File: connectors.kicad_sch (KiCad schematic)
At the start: 4 parts, among them J1 Conn_01x04_Pin, J2 Conn_01x04_Pin, J3 Conn_01x09_Pin, J4 Conn_02x03_Odd_Even

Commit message: Assigned footprints to symbols
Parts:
- J1, J2: footprint (none) -> Connector_PinHeader_2.54mm:PinHeader_1x04_P2.54mm_Vertical
- J3: footprint (none) -> Connector_PinHeader_2.54mm:PinHeader_1x09_P2.54mm_Vertical
- J4: footprint (none) -> Connector_PinHeader_2.54mm:PinHeader_2x03_P2.54mm_Vertical
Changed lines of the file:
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@@
       (effects (font (size 1.27 1.27)))
     )
-    (property "Footprint" "" (at 102.87 105.41 0)
+    (property "Footprint" "Connector_PinHeader_2.54mm:PinHeader_1x09_P2.54mm_Vertical" (at 102.87 105.41 0)
       (effects (font (size 1.27 1.27)) hide)
     )
@@
       (effects (font (size 1.27 1.27)))
     )
-    (property "Footprint" "" (at 101.6 71.12 0)
+    (property "Footprint" "Connector_PinHeader_2.54mm:PinHeader_1x04_P2.54mm_Vertical" (at 101.6 71.12 0)
       (effects (font (size 1.27 1.27)) hide)
     )
@@
       (effects (font (size 1.27 1.27)))
     )
-    (property "Footprint" "" (at 127 71.12 0)
+    (property "Footprint" "Connector_PinHeader_2.54mm:PinHeader_1x04_P2.54mm_Vertical" (at 127 71.12 0)
       (effects (font (size 1.27 1.27)) hide)
     )
@@
       (effects (font (size 1.27 1.27)))
     )
-    (property "Footprint" "" (at 130.81 104.14 0)
+    (property "Footprint" "Connector_PinHeader_2.54mm:PinHeader_2x03_P2.54mm_Vertical" (at 130.81 104.14 0)
       (effects (font (size 1.27 1.27)) hide)
     )

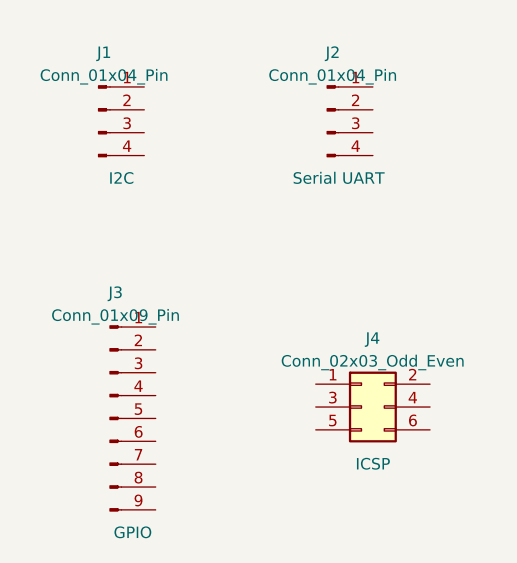
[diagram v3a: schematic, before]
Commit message: completed writing of embedded connector sheet
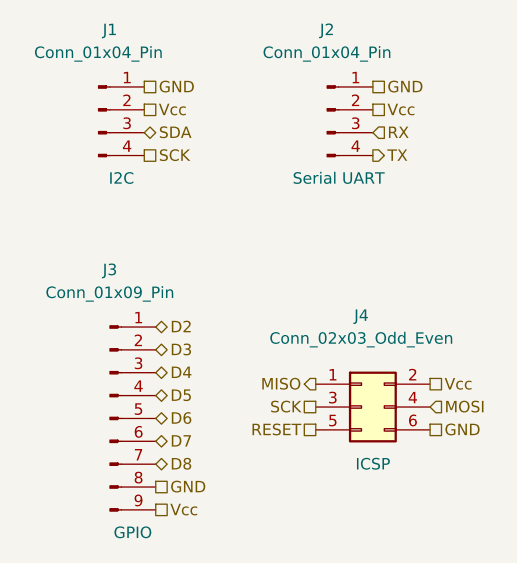
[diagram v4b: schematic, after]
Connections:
- net D2: now reaches J3.1 (Pin_1)
- net D3: now reaches J3.2 (Pin_2)
- net D4: now reaches J3.3 (Pin_3)
- net D5: now reaches J3.4 (Pin_4)
- net D6: now reaches J3.5 (Pin_5)
- net D7: now reaches J3.6 (Pin_6)
- net D8: now reaches J3.7 (Pin_7)
- net GND: now reaches J3.8 (Pin_8)
- net GND: now also J1.1 (Pin_1), J2.1 (Pin_1), J4.6 (Pin_6)
- net Vcc: now reaches J3.9 (Pin_9)
- net Vcc: now also J1.2 (Pin_2), J2.2 (Pin_2), J4.2 (Pin_2)
- net SDA: now reaches J1.3 (Pin_3)
- net SCK: now reaches J1.4 (Pin_4)
- net SCK: now also J4.3 (Pin_3)
- net RX: now reaches J2.3 (Pin_3)
- net TX: now reaches J2.4 (Pin_4)
- net MISO: now reaches J4.1 (Pin_1)
- net MOSI: now reaches J4.4 (Pin_4)
- net RESET: now reaches J4.5 (Pin_5)
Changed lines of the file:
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@@
 (kicad_sch (version 20230121) (generator eeschema)
   (paper "A4")
+  (hierarchical_label "Vcc" (shape passive) (at 106.68 71.12 0) (fields_autoplaced)
+    (effects (font (size 1.27 1.27)) (justify left))
+  )
+  (hierarchical_label "RESET" (shape passive) (at 125.73 106.68 180) (fields_autoplaced)
+    (effects (font (size 1.27 1.27)) (justify right))
+  )
+  (hierarchical_label "Vcc" (shape passive) (at 132.08 71.12 0) (fields_autoplaced)
+    (effects (font (size 1.27 1.27)) (justify left))
+  )
+  (hierarchical_label "GND" (shape passive) (at 132.08 68.58 0) (fields_autoplaced)
+    (effects (font (size 1.27 1.27)) (justify left))
+  )
+  (hierarchical_label "RX" (shape input) (at 132.08 73.66 0) (fields_autoplaced)
+    (effects (font (size 1.27 1.27)) (justify left))
+  )
+  (hierarchical_label "GND" (shape passive) (at 106.68 68.58 0) (fields_autoplaced)
+    (effects (font (size 1.27 1.27)) (justify left))
+  )
+  (hierarchical_label "D3" (shape bidirectional) (at 107.95 97.79 0) (fields_autoplaced)
+    (effects (font (size 1.27 1.27)) (justify left))
+  )
+  (hierarchical_label "GND" (shape passive) (at 138.43 106.68 0) (fields_autoplaced)
+    (effects (font (size 1.27 1.27)) (justify left))
+  )
+  (hierarchical_label "MISO" (shape output) (at 125.73 101.6 180) (fields_autoplaced)
+    (effects (font (size 1.27 1.27)) (justify right))
+  )
+  (hierarchical_label "D7" (shape bidirectional) (at 107.95 107.95 0) (fields_autoplaced)
+    (effects (font (size 1.27 1.27)) (justify left))
+  )
+  (hierarchical_label "D2" (shape bidirectional) (at 107.95 95.25 0) (fields_autoplaced)
+    (effects (font (size 1.27 1.27)) (justify left))
+  )
+  (hierarchical_label "SCK" (shape passive) (at 106.68 76.2 0) (fields_autoplaced)
+    (effects (font (size 1.27 1.27)) (justify left))
+  )
+  (hierarchical_label "SCK" (shape passive) (at 125.73 104.14 180) (fields_autoplaced)
+    (effects (font (size 1.27 1.27)) (justify right))
+  )
+  (hierarchical_label "SDA" (shape bidirectional) (at 106.68 73.66 0) (fields_autoplaced)
+    (effects (font (size 1.27 1.27)) (justify left))
+  )
+  (hierarchical_label "MOSI" (shape input) (at 138.43 104.14 0) (fields_autoplaced)
+    (effects (font (size 1.27 1.27)) (justify left))
+  )
+  (hierarchical_label "D5" (shape bidirectional) (at 107.95 102.87 0) (fields_autoplaced)
+    (effects (font (size 1.27 1.27)) (justify left))
+  )
+  (hierarchical_label "D8" (shape bidirectional) (at 107.95 110.49 0) (fields_autoplaced)
+    (effects (font (size 1.27 1.27)) (justify left))
+  )
+  (hierarchical_label "TX" (shape output) (at 132.08 76.2 0) (fields_autoplaced)
+    (effects (font (size 1.27 1.27)) (justify left))
+  )
+  (hierarchical_label "Vcc" (shape passive) (at 138.43 101.6 0) (fields_autoplaced)
+    (effects (font (size 1.27 1.27)) (justify left))
+  )
+  (hierarchical_label "Vcc" (shape passive) (at 107.95 115.57 0) (fields_autoplaced)
+    (effects (font (size 1.27 1.27)) (justify left))
+  )
+  (hierarchical_label "D6" (shape bidirectional) (at 107.95 105.41 0) (fields_autoplaced)
+    (effects (font (size 1.27 1.27)) (justify left))
+  )
+  (hierarchical_label "D4" (shape bidirectional) (at 107.95 100.33 0) (fields_autoplaced)
+    (effects (font (size 1.27 1.27)) (justify left))
+  )
+  (hierarchical_label "GND" (shape passive) (at 107.95 113.03 0) (fields_autoplaced)
+    (effects (font (size 1.27 1.27)) (justify left))
+  )
   (symbol (lib_id "Connector:Conn_01x09_Pin") (at 102.87 105.41 0) (unit 1)
     (in_bom yes) (on_board yes) (dnp no)
-    (property "Reference" "J3" (at 103.505 91.44 0)
+    (property "Reference" "J3" (at 102.87 88.9 0)
       (effects (font (size 1.27 1.27)))
     )
-    (property "Value" "Conn_01x09_Pin" (at 103.505 93.98 0)
+    (property "Value" "Conn_01x09_Pin" (at 102.87 91.44 0)
       (effects (font (size 1.27 1.27)))
     )
@@
   (symbol (lib_id "Connector:Conn_01x04_Pin") (at 101.6 71.12 0) (unit 1)
     (in_bom yes) (on_board yes) (dnp no)
-    (property "Reference" "J1" (at 102.235 64.77 0)
+    (property "Reference" "J1" (at 102.87 62.23 0)
       (effects (font (size 1.27 1.27)))
     )
-    (property "Value" "Conn_01x04_Pin" (at 102.235 67.31 0)
+    (property "Value" "Conn_01x04_Pin" (at 101.6 64.77 0)
       (effects (font (size 1.27 1.27)))
     )
@@
   (symbol (lib_id "Connector:Conn_01x04_Pin") (at 127 71.12 0) (unit 1)
     (in_bom yes) (on_board yes) (dnp no)
-    (property "Reference" "J2" (at 127.635 64.77 0)
+    (property "Reference" "J2" (at 127 62.23 0)
       (effects (font (size 1.27 1.27)))
     )
-    (property "Value" "Conn_01x04_Pin" (at 127.635 67.31 0)
+    (property "Value" "Conn_01x04_Pin" (at 127 64.77 0)
       (effects (font (size 1.27 1.27)))
     )
@@
   (symbol (lib_id "Connector_Generic:Conn_02x03_Odd_Even") (at 130.81 104.14 0) (unit 1)
     (in_bom yes) (on_board yes) (dnp no)
-    (property "Reference" "J4" (at 132.08 96.52 0)
+    (property "Reference" "J4" (at 130.81 93.98 0)
       (effects (font (size 1.27 1.27)))
     )
-    (property "Value" "Conn_02x03_Odd_Even" (at 132.08 99.06 0)
+    (property "Value" "Conn_02x03_Odd_Even" (at 130.81 96.52 0)
       (effects (font (size 1.27 1.27)))
     )
